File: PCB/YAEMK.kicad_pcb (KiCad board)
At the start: 2 copper layers, 162.8 x 130.8 mm, 178 parts, among them J1 DBG, P1 PC, P2 Link, P3 SSD1107, Q1 SSP6206, Q2 Q_PNP_BCE, SW1 ALPS EC11, U1 USBLC6-2SC6, U2 USBLC6-2SC6, U3 STM32F103CBTx, U4 24LC64

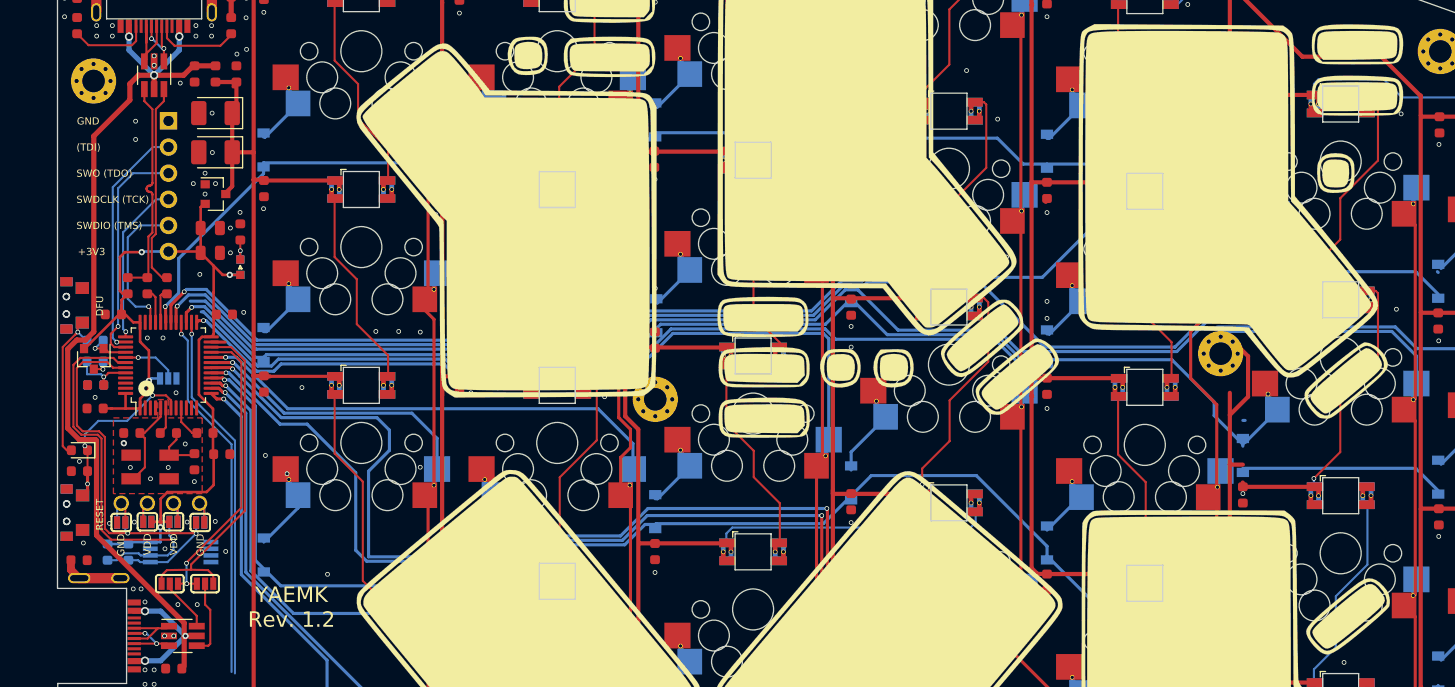
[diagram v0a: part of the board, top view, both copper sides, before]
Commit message: Update YAEMK 1
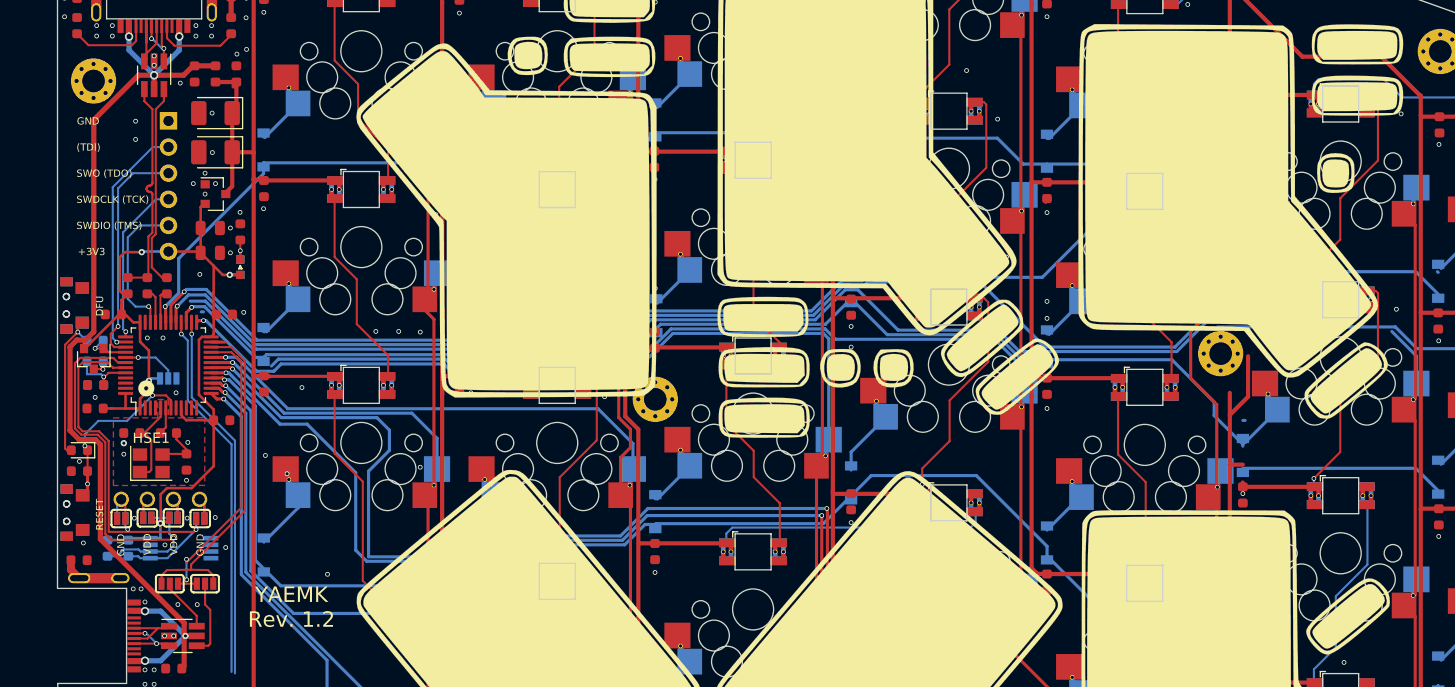
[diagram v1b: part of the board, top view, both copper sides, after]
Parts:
- removed L2: 600Ω @ 100MHz 1A, prettylib:SMD-0603
- HSE1: footprint prettylib:Crystal_SMD_EuroQuartz_MJ-4Pin_5.0x3.2mm -> Crystal:Crystal_SMD_3225-4Pin_3.2x2.5mm
- moved C47 3.30 mm to (93.1, 81.3)
- moved C59 0.78 mm to (89.7, 85.3)
- moved JP10 0.38 mm to (91.0, 90.8)
- moved JP3 0.38 mm to (91.0, 90.8)
- moved JP4 0.38 mm to (88.4, 90.8)
- moved JP5 0.38 mm to (85.9, 90.8)
- moved JP6 0.38 mm to (83.3, 90.8)
- moved JP7 0.38 mm to (83.3, 90.8)
- moved JP8 0.38 mm to (85.9, 90.8)
- moved JP9 0.38 mm to (88.4, 90.8)
- moved P3 0.38 mm to (96.7, 90.4)
- moved R14 0.38 mm to (82.0, 93.7)
- moved R9 0.38 mm to (84.0, 93.7)
- moved U4 0.38 mm to (89.1, 93.7)
- moved HSE1 0.37 mm to (86.2, 85.5)
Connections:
- U3 pad 9: Net-(L2-Pad1) -> VDD
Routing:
- net Col7: track 191.3 -> 174.5 mm
- net Col5: track 179.6 -> 170.8 mm
- net VDD: track 89.0 -> 92.6 mm
- net Net-(L2-Pad1): track 3.40 -> 0.00 mm
- net +5V: track 1018.0 -> 1015.5 mm
- net HSE_IN: track 9.15 -> 8.65 mm
- net VSS: vias 130 -> 127
